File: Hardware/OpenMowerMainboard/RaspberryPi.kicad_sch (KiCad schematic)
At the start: 8 parts, among them J16 Conn_02x03_Odd_Even, J4 RPi_GPIO, M1 Fan, Q3 BSS138, U3 SIP32509DT

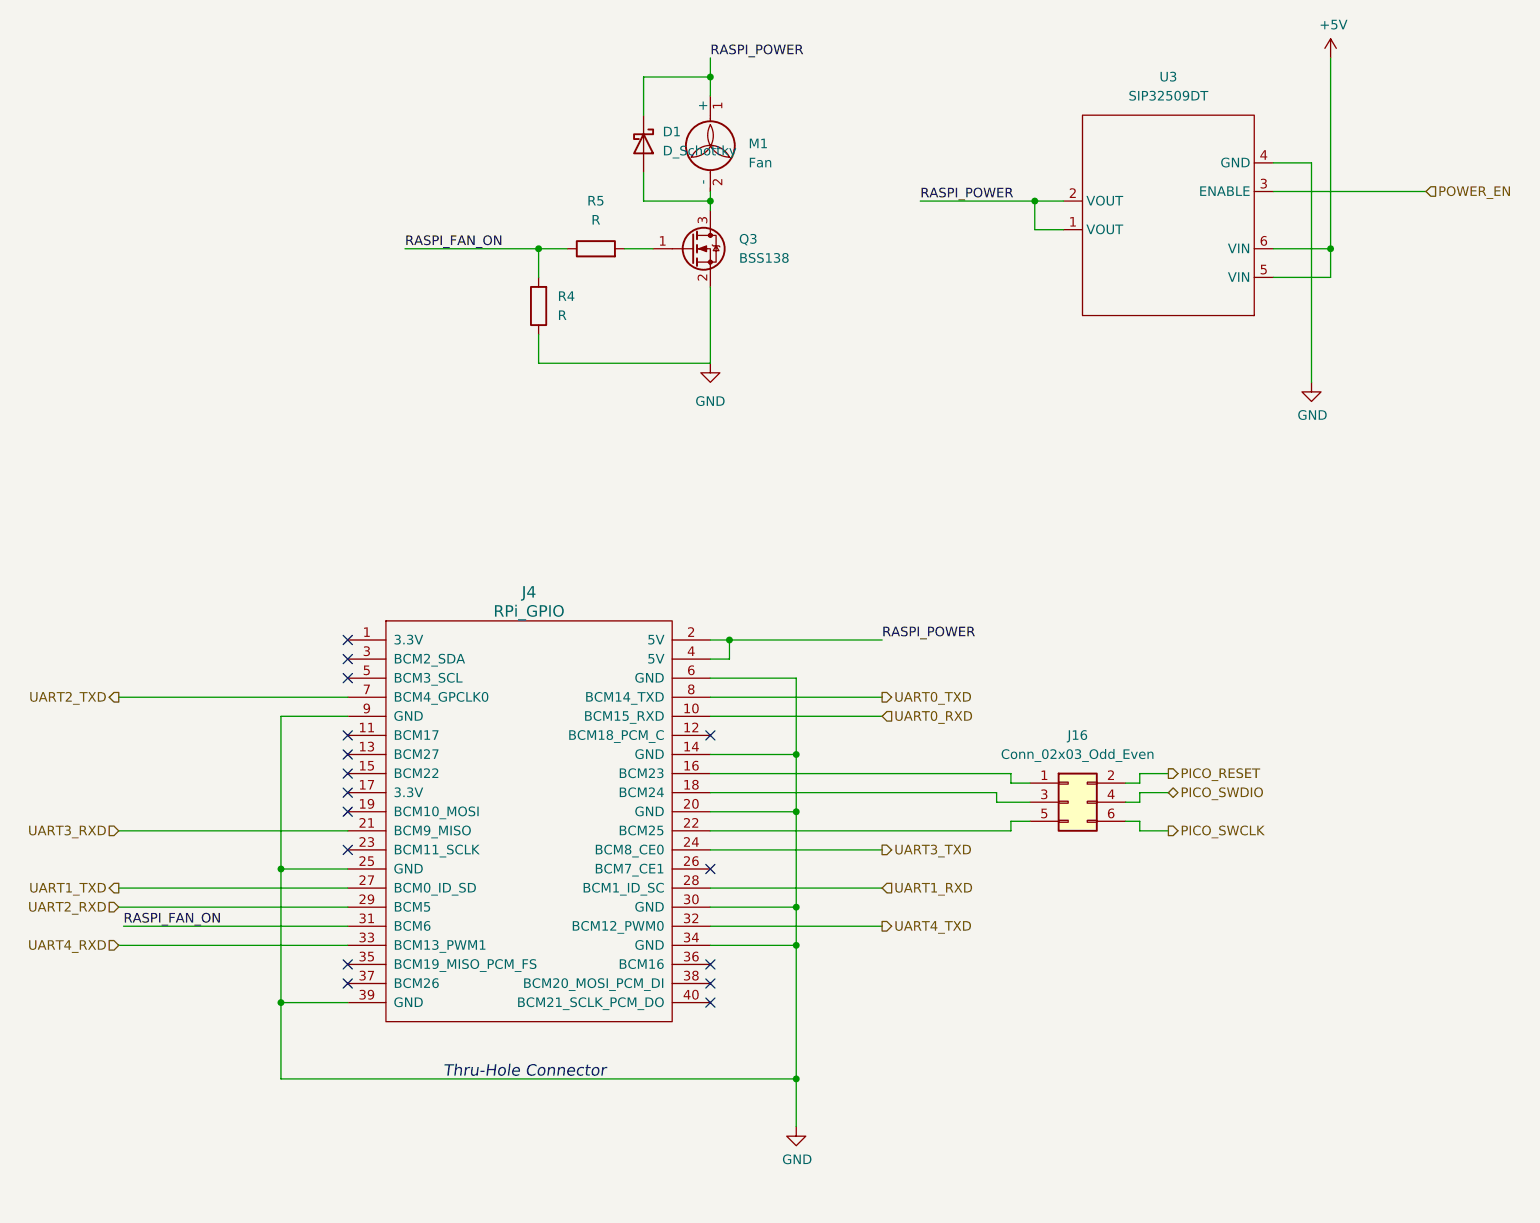
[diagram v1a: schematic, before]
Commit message: added footprints to schematic
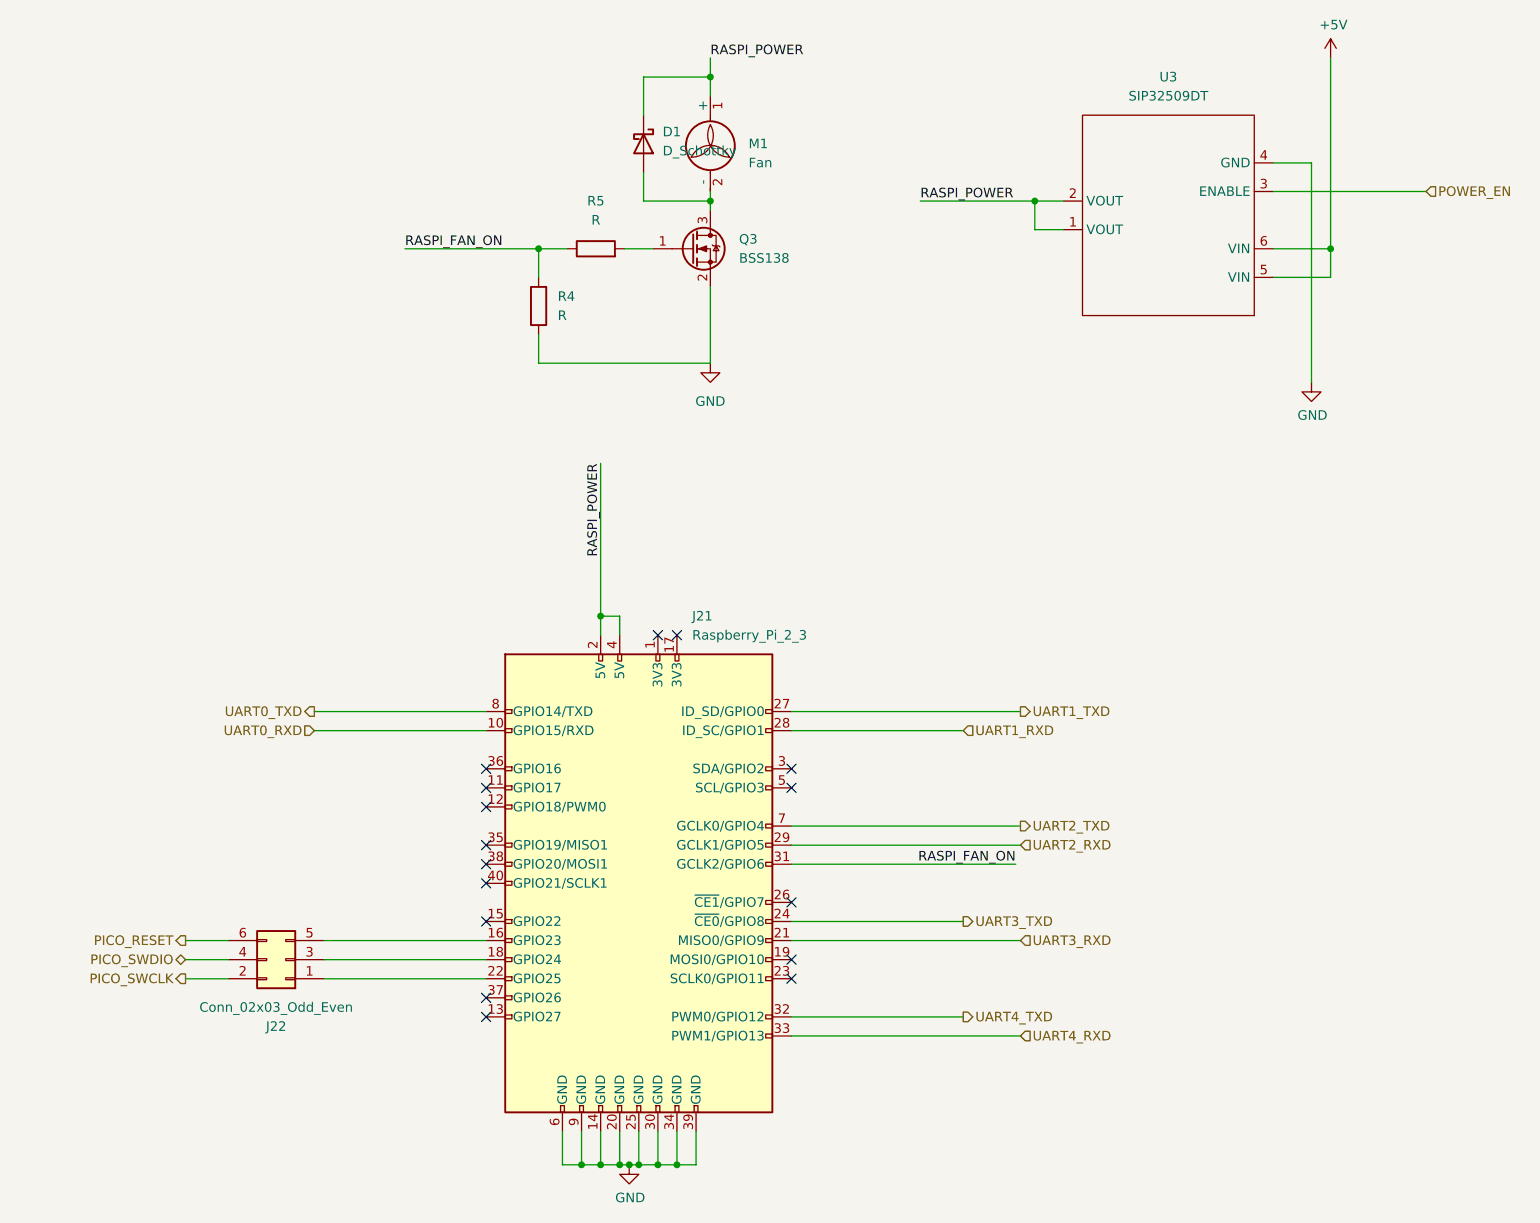
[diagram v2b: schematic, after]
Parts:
- removed J16: Conn_02x03_Odd_Even, Connector_PinHeader_2.54mm:PinHeader_2x03_P2.54mm_Vertical, symbol Connector_Generic:Conn_02x03_Odd_Even
- removed J4: RPi_GPIO, Connector_PinSocket_2.54mm:PinSocket_2x20_P2.54mm_Vertical_SMD, symbol OpenMowerMainboard-rescue:RPi_GPIO-RPi_Hat
- added J21: Raspberry_Pi_2_3, Connector_PinSocket_2.54mm:PinSocket_2x20_P2.54mm_Vertical_SMD, symbol Connector:Raspberry_Pi_2_3
- added J22: Conn_02x03_Odd_Even, Connector_PinHeader_2.54mm:PinHeader_2x03_P2.54mm_Vertical, symbol Connector_Generic:Conn_02x03_Odd_Even
- D1: footprint (none) -> Diode_SMD:D_SOD-123F
- M1: footprint (none) -> Connector_JST:JST_XH_B2B-XH-A_1x02_P2.50mm_Vertical
- R4, R5: footprint Resistor_SMD:R_0805_2012Metric -> Resistor_SMD:R_0805_2012Metric_Pad1.20x1.40mm_HandSolder
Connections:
- net GND: now also J21.14 (GND), J21.20 (GND), J21.25 (GND), J21.30 (GND), J21.34 (GND), J21.39 (GND), J21.6 (GND), J21.9 (GND)
- net PICO_RESET: now also J22.6 (Pin_6)
- net PICO_SWCLK: now also J22.2 (Pin_2)
- net PICO_SWDIO: now also J22.4 (Pin_4)
- net RASPI_FAN_ON: now also J21.31 (GCLK2/GPIO6)
- net RASPI_POWER: now also J21.2 (5V), J21.4 (5V)
- net UART0_RXD: now also J21.10 (GPIO15/RXD)
- net UART0_TXD: now also J21.8 (GPIO14/TXD)
- net UART1_RXD: now also J21.28 (ID_SC/GPIO1)
- net UART1_TXD: now also J21.27 (ID_SD/GPIO0)
- net UART2_RXD: now also J21.29 (GCLK1/GPIO5)
- net UART2_TXD: now also J21.7 (GCLK0/GPIO4)
- net UART3_RXD: now also J21.21 (MISO0/GPIO9)
- net UART3_TXD: now also J21.24 (~{CE0}/GPIO8)
- net UART4_RXD: now also J21.33 (PWM1/GPIO13)
- net UART4_TXD: now also J21.32 (PWM0/GPIO12)
- new net: J21.22 (GPIO25), J22.1 (Pin_1)
- new net: J21.18 (GPIO24), J22.3 (Pin_3)
- new net: J21.16 (GPIO23), J22.5 (Pin_5)
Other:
- note removed: "Thru-Hole Connector"

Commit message: wip
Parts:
- M1: footprint Connector_JST:JST_XH_B2B-XH-A_1x02_P2.50mm_Vertical -> Connector_PinHeader_2.54mm:PinHeader_1x02_P2.54mm_Vertical
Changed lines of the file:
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@@
       (effects (font (size 1.27 1.27)) (justify left))
     )
-    (property "Footprint" "Connector_JST:JST_XH_B2B-XH-A_1x02_P2.50mm_Vertical" (id 2) (at 116.84 36.576 0)
+    (property "Footprint" "Connector_PinHeader_2.54mm:PinHeader_1x02_P2.54mm_Vertical" (id 2) (at 116.84 36.576 0)
       (effects (font (size 1.27 1.27)) hide)
     )
